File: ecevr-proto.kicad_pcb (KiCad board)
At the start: 4 copper layers, 100 x 92 mm, 395 parts, among them J1 PEN_SEL, J19 SFP, J2 PEN_SEL, J20 SFP_CAGE, J2001 BNC, J2051 BNC, J2201 BEL_0845_2G1T_H5, J3 USB_C_Receptacle_USB2.0, J4 JTAG, SW1 PROG, SW2101 SW_DIP_x08, U1 XC7A35T-CSG325, U10 74LVC1G02, U11 UTC2000, U12 5P49V6965, U2 AT25SL641, U2001 74LVC2T45DC, U2051 74LVC2T45DC, U2101 74AHC1T86, U2102 74AHC1T86, U2103 PCA9306, U2104 24AA0x, U2105 74AHC1T86, U2106 74AHC1T86, U2201 74AHC1T86, U2202 74LVC1G06, U2301 lan9254, U2302 SN74LV1T34DBV, U3 FT240XQ, U4 TLV62569ADDC, U5 TPS62A01A-SOT563, U6 TPS62A01A-SOT563, U7 TLV62569ADDC, U8 74ALVC125, U9 TLV62569ADDC, X2301 FNETHE025, Y1 25MHz

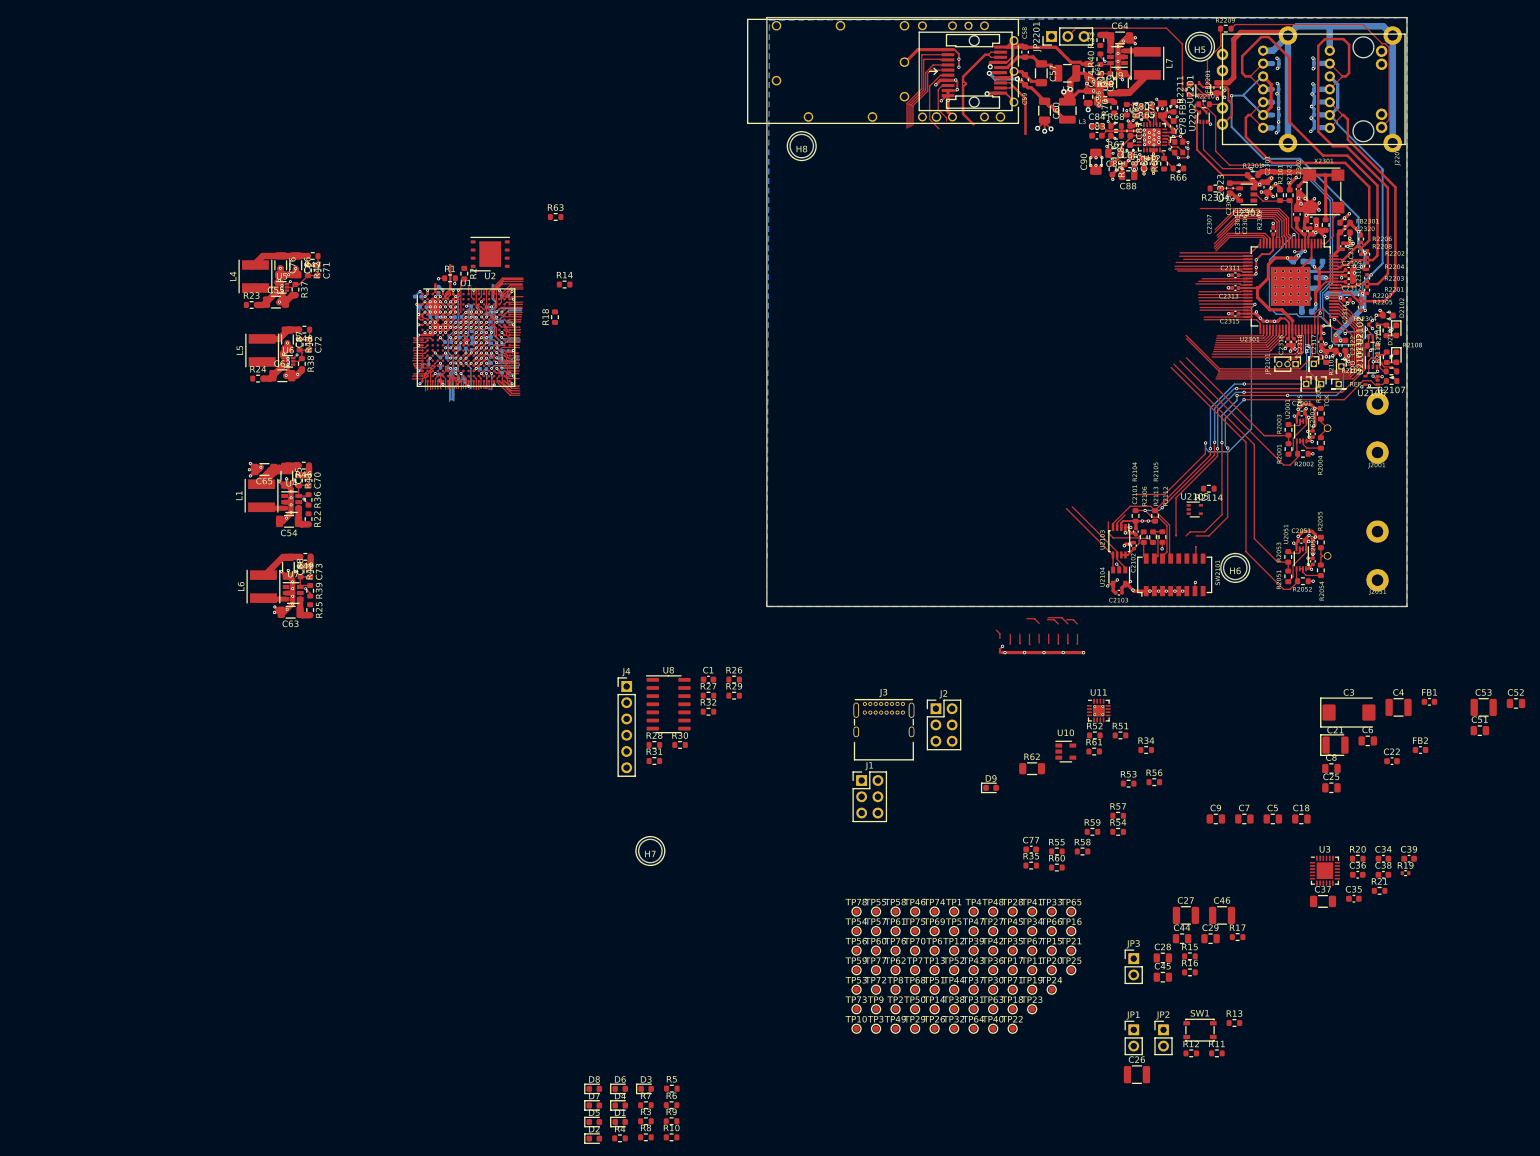
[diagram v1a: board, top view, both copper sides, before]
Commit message: WIP: point before we change to OSH/relaxed process
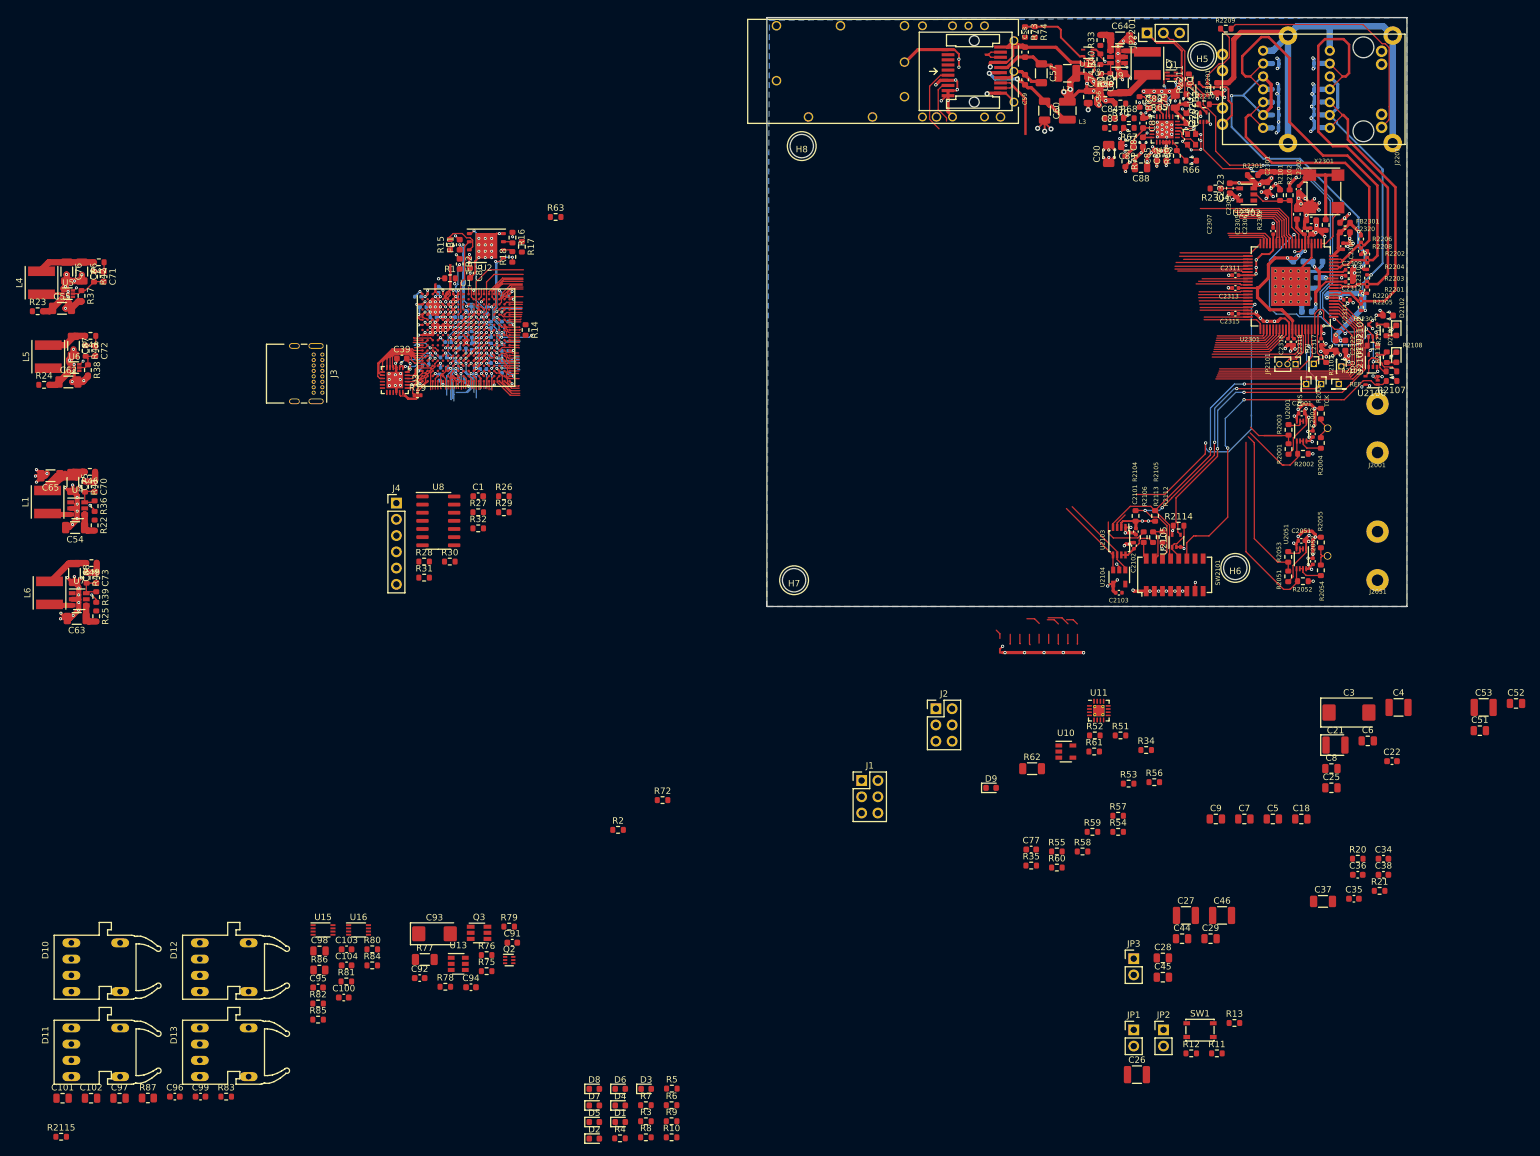
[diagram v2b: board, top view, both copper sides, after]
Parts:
- removed TP1, TP10, TP11, TP12, TP13, TP14, TP15, TP16, TP17, TP18, TP19, TP2, TP20, TP21, TP22, TP23, TP24, TP25, TP26, TP27, TP28, TP29, TP3, TP30, TP31, TP32, TP33, TP34, TP35, TP36, TP37, TP38, TP39, TP4, TP40, TP41, TP42, TP43, TP44, TP45, TP46, TP47, TP48, TP49, TP5, TP50, TP51, TP52, TP53, TP54, TP55, TP56, TP57, TP58, TP59, TP6, TP60, TP61, TP62, TP63, TP64, TP65, TP66, TP67, TP68, TP69, TP7, TP70, TP71, TP72, TP73, TP74, TP75, TP76, TP77, TP78, TP8, TP9: TestPoint_Small, TestPoint:TestPoint_Pad_D1.0mm
- added C100: 100nF, Capacitor_SMD:C_0603_1608Metric, F.Cu at (33.9, 183.1)
- added C101: 1uF, Capacitor_SMD:C_0805_2012Metric, F.Cu at (-10.0, 198.8)
- added C102: 1uF, Capacitor_SMD:C_0805_2012Metric, F.Cu at (-5.58, 198.8)
- added C103: 100nF, Capacitor_SMD:C_0603_1608Metric, F.Cu at (34.3, 175.6)
- added C104: 100nF, Capacitor_SMD:C_0603_1608Metric, F.Cu at (34.3, 178.1)
- added C91: 100n, Capacitor_SMD:C_0603_1608Metric, F.Cu at (60.2, 174.5)
- added C92: 100n, Capacitor_SMD:C_0603_1608Metric, F.Cu at (45.8, 180.1)
- added C93: 220u, Capacitor_Tantalum_SMD:CP_EIA-6032-28_Kemet-C, F.Cu at (48.1, 173.1)
- added C94: 1n, Capacitor_SMD:C_0603_1608Metric, F.Cu at (53.8, 181.5)
- added C95: 100nF, Capacitor_SMD:C_0603_1608Metric, F.Cu at (29.9, 181.5)
- added C96: 100nF, Capacitor_SMD:C_0603_1608Metric, F.Cu at (7.50, 198.6)
- added C97: 1uF, Capacitor_SMD:C_0805_2012Metric, F.Cu at (-1.14, 198.8)
- added C98: 1uF, Capacitor_SMD:C_0805_2012Metric, F.Cu at (30.1, 175.8)
- added C99: 100nF, Capacitor_SMD:C_0603_1608Metric, F.Cu at (11.5, 198.6)
- added D10: HFBR2528, proj_footprints:HFBR25XX, F.Cu at (-8.66, 178.4)
- added D11: HFBR1528, proj_footprints:HFBR25XX, F.Cu at (-8.66, 191.6)
- added D12: HFBR2528, proj_footprints:HFBR25XX, F.Cu at (11.4, 178.4)
- added D13: HFBR1528, proj_footprints:HFBR25XX, F.Cu at (11.4, 191.6)
- added Q1: SSM6N35AFE, proj_footprints:SOT-563-adjusted, F.Cu at (163.2, 39.1)
- added Q2: SSM6N35AFE, proj_footprints:SOT-563-adjusted, F.Cu at (59.7, 177.2)
- added Q3: Si3477, Package_TO_SOT_SMD:TSOT-23-6, F.Cu at (55.0, 173.0)
- added R2115: 10k, Resistor_SMD:R_0603_1608Metric, F.Cu at (-10.3, 204.8)
- added R72: 3k3, Resistor_SMD:R_0603_1608Metric, F.Cu at (83.7, 152.2)
- added R73: 10k, Resistor_SMD:R_0603_1608Metric, F.Cu at (140.3, 32.2)
- added R74: 10k, Resistor_SMD:R_0603_1608Metric, F.Cu at (141.8, 32.2)
- added R75: 100k, Resistor_SMD:R_0603_1608Metric, F.Cu at (56.2, 179.0)
- added R76: 100k, Resistor_SMD:R_0603_1608Metric, F.Cu at (56.2, 176.5)
- added R77: 47, Resistor_SMD:R_1206_3216Metric, F.Cu at (46.6, 177.2)
- added R78: 100k, Resistor_SMD:R_0603_1608Metric, F.Cu at (49.8, 181.4)
- added R79: 10k, Resistor_SMD:R_0603_1608Metric, F.Cu at (59.7, 172.0)
- added R80: 100k, Resistor_SMD:R_0603_1608Metric, F.Cu at (38.3, 175.6)
- added R81: 100k, Resistor_SMD:R_0603_1608Metric, F.Cu at (34.3, 180.6)
- added R82: 1k, Resistor_SMD:R_0603_1608Metric, F.Cu at (29.9, 184.0)
- added R83: 1k, Resistor_SMD:R_0603_1608Metric, F.Cu at (15.5, 198.6)
- added R84: 1k, Resistor_SMD:R_0603_1608Metric, F.Cu at (38.3, 178.1)
- added R85: 1k, Resistor_SMD:R_0603_1608Metric, F.Cu at (29.9, 186.5)
- added R86: 90, Resistor_SMD:R_0805_2012Metric, F.Cu at (30.1, 178.8)
- added R87: 90, Resistor_SMD:R_0805_2012Metric, F.Cu at (3.29, 198.8)
- added U13: TPS3808DBV, Package_TO_SOT_SMD:SOT-23-6, F.Cu at (51.8, 177.8)
- added U14: 74LVC1G06, proj_footprints:SOT-5x3, F.Cu at (150.2, 35.5)
- added U15: 74LVC2T45DC, Package_SO:VSSOP-8_2.3x2mm_P0.5mm, F.Cu at (30.7, 172.5)
- added U16: 74LVC2T45DC, Package_SO:VSSOP-8_2.3x2mm_P0.5mm, F.Cu at (36.2, 172.5)
- C83, C84: value C_Small -> 100n
- J1: value PEN_SEL -> CUR_SEL
- R2: value 50 -> 3k3
- R64, R65: value 10k -> 3k3
- U10: value 74LVC1G02 -> 74VHC1G03
- moved C39 175.7 mm to (43.0, 83.2)
- moved R19 171.5 mm to (45.4, 89.0)
- moved FB2 168.2 mm to (52.0, 68.5), turned to 270 degrees
- moved FB1 167.5 mm to (52.0, 65.5), turned to 90 degrees
- moved U3 164.3 mm to (41.9, 86.6), turned to 270 degrees
- moved R15 160.4 mm to (50.5, 65.5), turned to 90 degrees
- moved R16 156.1 mm to (60.2, 64.4), turned to 270 degrees
- moved R17 155.4 mm to (61.7, 65.8), turned to 270 degrees
- moved C86 104.4 mm to (53.6, 69.9), turned to 270 degrees
- moved J3 100.8 mm to (30.6, 82.7), turned to 270 degrees
- moved R2 90.2 mm to (76.8, 156.9), turned to 0 degrees
- moved H7 47.9 mm to (104.2, 117.9)
- moved C1 46.0 mm to (54.9, 104.8)
- moved J4 46.0 mm to (42.1, 105.8)
- moved R26 46.0 mm to (58.9, 104.8)
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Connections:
- net /USB, SDIO, RJ45, JTAG, UART, I2C/USBD_N renamed /USB, JTAG, I2C/USBD_N
- net /USB, SDIO, RJ45, JTAG, UART, I2C/USBD_P renamed /USB, JTAG, I2C/USBD_P
- C86 pad 1: GND -> +1V8
- C86 pad 2: +1V8 -> GND
- J19 pad 2: B13_L6_P -> IO_L7N_T1_AD2N_15
- J19 pad 3: B13_L6_N -> /SFP Connector/TX_DISABLE
- J19 pad 4: SDA1 -> SDA1_3V3
- J19 pad 5: SCL1 -> SCL1_3V3
- J19 pad 6: B13_L4_P -> IO_L5N_T0_AD9N_15
- J19 pad 8: B13_L4_N -> IO_L4N_T0_15
- J2 pad 4: USB_PWRENb -> IO_L15N_T2_DQS_34
- R10 pad 1: B13_L18_P -> IO_L20P_T3_34
- R19 pad 1: FIFO_CLK -> IO_L12P_T1_MRCC_34
- R2 pad 1: /fpga/fpga_bank0_cfg/CCLK -> +1V8
- R2 pad 2: Net-(R2-Pad2) -> IO_L23N_T3_A02_D18_14
- R2001 pad 2: B35_L10_P -> IO_L18N_T2_A11_D27_14
- R2002 pad 1: B35_L20_N -> IO_L13N_T2_MRCC_14
- R2003 pad 1: B35_L10_P -> IO_L18N_T2_A11_D27_14
- R2051 pad 2: B35_L20_P -> IO_L18P_T2_A12_D28_14
- R2052 pad 1: B35_L25 -> IO_L17N_T2_A13_D29_14
- R2053 pad 1: B35_L20_P -> IO_L18P_T2_A12_D28_14
- R2106 pad 1: B35_L3_N -> IO_L3N_T0_DQS_EMCCLK_14
- R2112 pad 1: Net-(R2112-Pad1) -> IO_L21P_T3_DQS_14
- R2113 pad 2: Net-(R2112-Pad1) -> IO_L21P_T3_DQS_14
- R2114 pad 2: Net-(R2114-Pad2) -> IO_L22P_T3_A05_D21_14
- R3 pad 1: B13_L15_N -> IO_L3P_T0_DQS_34
- R4 pad 1: B13_L15_P -> IO_L3N_T0_DQS_34
- R5 pad 1: B13_L20_P -> IO_L18N_T2_34
- R53 pad 1: Net-(J1-Pad1) -> +5V
- R53 pad 2: +5V -> Net-(J1-Pad1)
- R6 pad 1: B13_L20_N -> IO_L18P_T2_34
- R62 pad 2: VBUS -> Net-(Q3-Pad1)
- R64 pad 1: I2C_SCL -> IO_L7P_T1_AD2P_15
- R65 pad 1: I2C_SDA -> IO_L8P_T1_AD10P_15
- R7 pad 1: B13_L21_P -> IO_25_34
- R8 pad 1: B13_L21_N -> IO_L20N_T3_34
- R9 pad 1: B13_L18_N -> IO_L23N_T3_34
- SW2101 pad 10: Net-(SW2101-Pad10) -> IO_L21N_T3_DQS_A06_D22_14
- SW2101 pad 12: Net-(R2114-Pad2) -> IO_L22P_T3_A05_D21_14
- SW2101 pad 15: Net-(R2112-Pad1) -> IO_L21P_T3_DQS_14
- SW2101 pad 7: Net-(SW2101-Pad7) -> GND
- SW2101 pad 8: Net-(SW2101-Pad8) -> GND
- SW2101 pad 9: Net-(SW2101-Pad9) -> IO_L22N_T3_A04_D20_14
- U1 pad E8: Net-(R2-Pad2) -> /fpga/fpga_bank0_cfg/CCLK
- U12 pad 8: I2C_SDA -> IO_L8P_T1_AD10P_15
- U12 pad 9: I2C_SCL -> IO_L7P_T1_AD2P_15
- U2001 pad 5: B35_L20_N -> IO_L13N_T2_MRCC_14
- U2051 pad 5: B35_L25 -> IO_L17N_T2_A13_D29_14
- U2103 pad 5: SDA0 -> IO_L23N_T3_A02_D18_14
- U2103 pad 6: SCL0 -> IO_L23P_T3_A03_D19_14
- U2104 pad 1: SCL0 -> IO_L23P_T3_A03_D19_14
- U2104 pad 3: SDA0 -> IO_L23N_T3_A02_D18_14
- U2104 pad 5: GND -> IO_25_14
- U2105 pad 1: Net-(R2114-Pad2) -> IO_L22P_T3_A05_D21_14
- U2301 pad 10: B34_L15_N -> IO_L8N_T1_AD10N_15
- U2301 pad 11: B34_L15_P -> IO_L9N_T1_DQS_AD3N_15
- U2301 pad 12: B34_L18_N -> IO_L10N_T1_AD11N_15
- U2301 pad 13: B34_L2_P -> IO_L13N_T2_MRCC_15
- U2301 pad 14: B34_L2_N -> IO_L15P_T2_DQS_15
- U2301 pad 15: B34_L12_P -> IO_L15N_T2_DQS_ADV_B_15
- U2301 pad 17: B34_L6_N -> IO_L16P_T2_A28_15
- U2301 pad 18: B34_L6_P -> IO_L16N_T2_A27_15
- U2301 pad 19: B34_L8_P -> IO_L18P_T2_A24_15
- U2301 pad 20: B35_L16_P -> IO_L18N_T2_A23_15
- U2301 pad 21: B35_L16_N -> IO_L14N_T2_SRCC_15
- U2301 pad 22: B34_L7_N -> IO_L13P_T2_MRCC_15
- U2301 pad 23: B35_L18_N -> IO_L17N_T2_A25_15
- U2301 pad 24: B35_L18_P -> IO_L17P_T2_A26_15
- U2301 pad 25: B35_L21_P -> IO_L24N_T3_RS0_15
- U2301 pad 26: B35_L15_N -> IO_L14P_T2_SRCC_15
- U2301 pad 28: B35_L15_P -> IO_L19N_T3_A21_VREF_15
- U2301 pad 29: B35_L8_P -> IO_L24P_T3_RS1_15
- U2301 pad 30: B35_L13_P -> IO_L19P_T3_A22_15
- U2301 pad 32: B35_L13_N -> IO_L23N_T3_FWE_B_15
- U2301 pad 33: B35_L11_N -> IO_L20N_T3_A19_15
- U2301 pad 34: B35_L14_P -> IO_L2N_T0_D03_14
- U2301 pad 35: B35_L14_N -> IO_L23P_T3_FOE_B_15
- U2301 pad 36: B35_L3_N -> IO_L3N_T0_DQS_EMCCLK_14
- U2301 pad 37: B35_L12_P -> IO_L8P_T1_D11_14
- U2301 pad 38: B35_L12_N -> IO_L4P_T0_D04_14
- U2301 pad 40: B35_L7_N -> IO_L4N_T0_D05_14
- U2301 pad 41: B35_L23_N -> IO_L7P_T1_D09_14
- U2301 pad 42: B35_L23_P -> IO_L7N_T1_D10_14
- U2301 pad 43: B35_L4_P -> IO_L10P_T1_D14_14
- U2301 pad 44: B35_L2_N -> IO_L6N_T0_D08_VREF_14
- U2301 pad 45: B35_L2_P -> IO_L9P_T1_DQS_14
- U2301 pad 46: B35_L5_N -> IO_L8N_T1_D12_14
- U2301 pad 47: B35_L17_P -> IO_L10N_T1_D15_14
- U2301 pad 48: B35_L17_N -> IO_L11P_T1_SRCC_14
- U2301 pad 49: B35_L6_N -> IO_L9N_T1_DQS_D13_14
- U2301 pad 52: B35_L24_P -> IO_L15P_T2_DQS_RDWR_B_14
- U2301 pad 53: B35_L24_N -> IO_L12N_T1_MRCC_14
- U2301 pad 57: B35_L0 -> IO_L11N_T1_SRCC_14
- U2301 pad 62: B35_L9_N -> IO_L14P_T2_SRCC_14
- U2301 pad 63: B35_L9_P -> IO_L15N_T2_DQS_DOUT_CSO_B_14
- U2301 pad 64: B35_L22_N -> IO_L14N_T2_SRCC_14
- U2301 pad 65: B35_L22_P -> IO_L16P_T2_CSI_B_14
- U2301 pad 66: B35_L10_N -> IO_L16N_T2_A15_D31_14
- U3 pad 1: FIFO_D1 -> IO_L12N_T1_MRCC_34
- U3 pad 17: FIFO_TXF -> IO_L16N_T2_34
- U3 pad 18: FIFO_RXE -> IO_L15P_T2_DQS_34
- U3 pad 19: FIFO_CLK -> IO_L12P_T1_MRCC_34
- U3 pad 2: FIFO_D7 -> IO_L11P_T1_SRCC_34
- U3 pad 20: USB_PWRENb -> IO_L15N_T2_DQS_34
- U3 pad 21: FIFO_D0 -> IO_L14N_T2_SRCC_34
- U3 pad 22: FIFO_D4 -> IO_L14P_T2_SRCC_34
- U3 pad 23: FIFO_D2 -> IO_L13N_T2_MRCC_34
- U3 pad 4: FIFO_D5 -> IO_L13P_T2_MRCC_34
- U3 pad 5: FIFO_D6 -> IO_L9N_T1_DQS_34
- U3 pad 6: FIFO_D3 -> IO_L11N_T1_SRCC_34
- U3 pad 7: FIFO_SIWU -> IO_L9P_T1_DQS_34
- U3 pad 8: FIFO_RDb -> IO_L7P_T1_34
- U3 pad 9: FIFO_WRb -> IO_L7N_T1_34
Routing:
- net B35_L3_N: track 61.6 -> 0.00 mm, vias 2 -> 0
- net IO_L3N_T0_DQS_EMCCLK_14: track 1.60 -> 63.2 mm, vias 0 -> 2
- net B35_L25: track 47.1 -> 0.00 mm
- net /lan9254/LINKACT0: track 112.3 -> 66.4 mm, vias 5 -> 2
- net B35_L20_P: track 40.8 -> 0.00 mm
- net B35_L9_N: track 38.4 -> 0.00 mm
- net IO_L16N_T2_A15_D31_14: track 3.29 -> 40.0 mm
- net B35_L10_N: track 36.7 -> 0.00 mm
- net IO_L16P_T2_CSI_B_14: track 3.09 -> 38.5 mm
- net B35_L22_P: track 35.4 -> 0.00 mm
- net IO_L14N_T2_SRCC_14: track 2.99 -> 37.0 mm
- net B35_L22_N: track 34.0 -> 0.00 mm
- net IO_L15N_T2_DQS_DOUT_CSO_B_14: track 1.50 -> 34.1 mm
- net B35_L9_P: track 32.6 -> 0.00 mm
- net IO_L14P_T2_SRCC_14: track 3.21 -> 34.8 mm
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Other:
- net class Default: clearance 0.0889 -> 0.1
- net class diffp: clearance 0.0889 -> 0.1; trace_width 0.0889 -> 0.1
- net class diffp_ec: clearance 0.0889 -> 0.1; trace_width 0.0889 -> 0.1
- rule trace_clearance: 0.0889 -> 0.1
- rule trace_min: 0.0889 -> 0.09
